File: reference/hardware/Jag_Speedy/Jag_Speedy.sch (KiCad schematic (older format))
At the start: 1 part, among them U3 Teensy 3.5

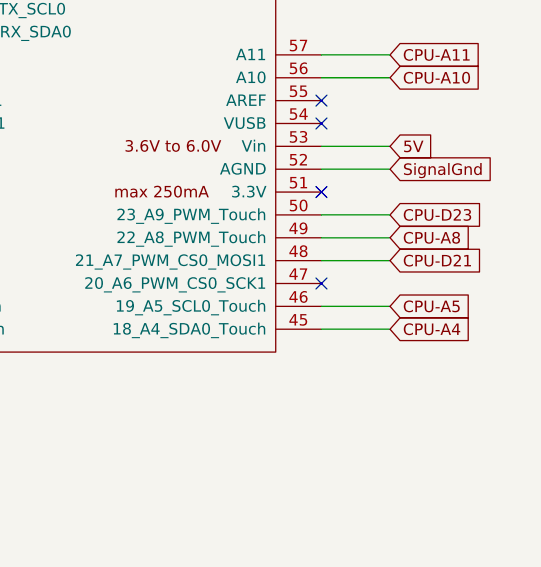
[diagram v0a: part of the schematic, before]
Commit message: EGR Input
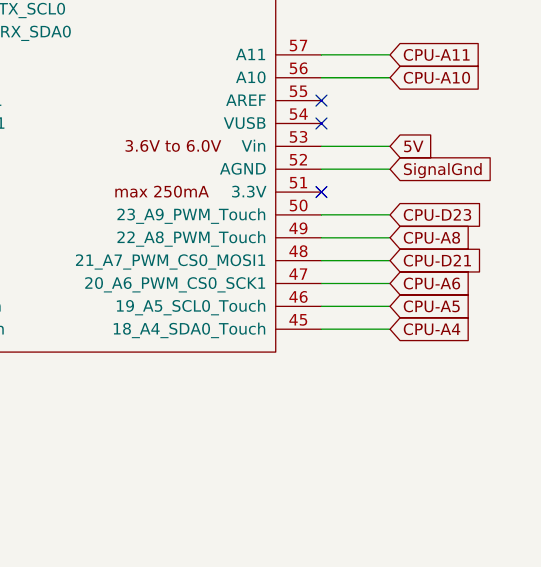
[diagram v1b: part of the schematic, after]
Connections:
- net CPU-A6: now reaches U3.47 (20_A6_PWM_CS0_SCK1)
- no-connect marks 39 -> 38
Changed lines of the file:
@@
 	1    0    0    -1
 $EndComp
-NoConn ~ 7200 5250
 NoConn ~ 4900 4150
 NoConn ~ 4900 4050
@@
 Wire Wire Line
 	4900 3250 4500 3250
+Text GLabel 7500 5250 2    50   Input ~ 0
+CPU-A6
+Wire Wire Line
+	7200 5250 7500 5250
 $EndSCHEMATC
